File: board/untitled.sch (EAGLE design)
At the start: 32 parts, among them IC1 PIC16F628P, IC2 LP2950CZ-3.3, Q1 BC546B, Q2 BC546B

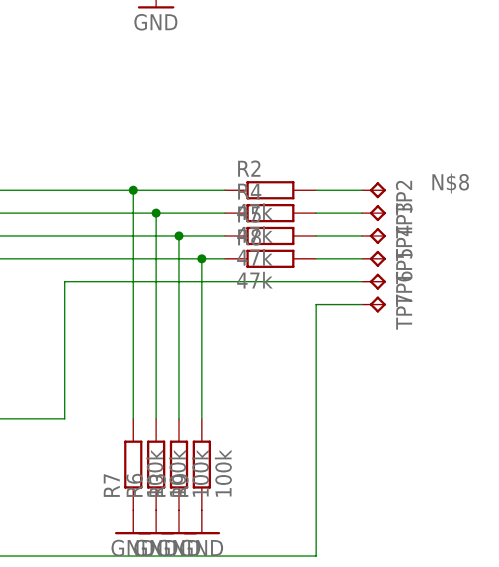
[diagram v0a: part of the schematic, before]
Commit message: - Added notes
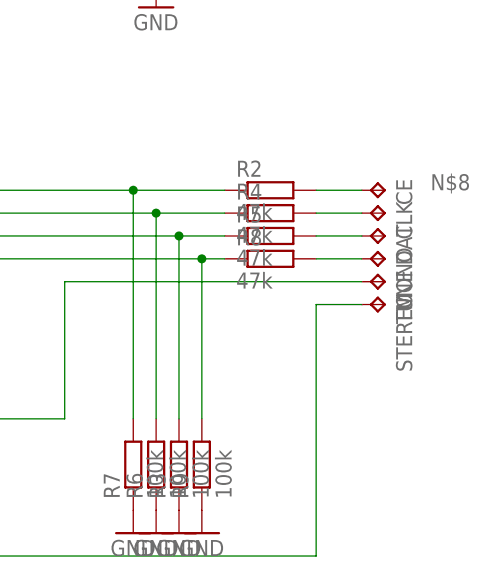
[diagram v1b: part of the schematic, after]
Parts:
- renumbered TP2 to CE, TP3 to CLK, TP4 to DAT, TP5 to MONO, TP6 to TUNE, TP7 to STEREO
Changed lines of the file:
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@@
 <part name="R13" library="rcl" library_urn="urn:adsk.eagle:library:334" deviceset="R-EU_" device="0204/7" package3d_urn="urn:adsk.eagle:package:23498/2" value="10k"/>
 <part name="P+3" library="supply1" library_urn="urn:adsk.eagle:library:371" deviceset="+5V" device=""/>
-<part name="TP2" library="testpad" library_urn="urn:adsk.eagle:library:385" deviceset="TP" device="B1,27" package3d_urn="urn:adsk.eagle:package:27944/2"/>
-<part name="TP3" library="testpad" library_urn="urn:adsk.eagle:library:385" deviceset="TP" device="B1,27" package3d_urn="urn:adsk.eagle:package:27944/2"/>
-<part name="TP4" library="testpad" library_urn="urn:adsk.eagle:library:385" deviceset="TP" device="B1,27" package3d_urn="urn:adsk.eagle:package:27944/2"/>
-<part name="TP5" library="testpad" library_urn="urn:adsk.eagle:library:385" deviceset="TP" device="B1,27" package3d_urn="urn:adsk.eagle:package:27944/2"/>
-<part name="TP6" library="testpad" library_urn="urn:adsk.eagle:library:385" deviceset="TP" device="B1,27" package3d_urn="urn:adsk.eagle:package:27944/2"/>
-<part name="TP7" library="testpad" library_urn="urn:adsk.eagle:library:385" deviceset="TP" device="B1,27" package3d_urn="urn:adsk.eagle:package:27944/2"/>
+<part name="CE" library="testpad" library_urn="urn:adsk.eagle:library:385" deviceset="TP" device="B1,27" package3d_urn="urn:adsk.eagle:package:27944/2"/>
+<part name="CLK" library="testpad" library_urn="urn:adsk.eagle:library:385" deviceset="TP" device="B1,27" package3d_urn="urn:adsk.eagle:package:27944/2"/>
+<part name="DAT" library="testpad" library_urn="urn:adsk.eagle:library:385" deviceset="TP" device="B1,27" package3d_urn="urn:adsk.eagle:package:27944/2"/>
+<part name="MONO" library="testpad" library_urn="urn:adsk.eagle:library:385" deviceset="TP" device="B1,27" package3d_urn="urn:adsk.eagle:package:27944/2"/>
+<part name="TUNE" library="testpad" library_urn="urn:adsk.eagle:library:385" deviceset="TP" device="B1,27" package3d_urn="urn:adsk.eagle:package:27944/2"/>
+<part name="STEREO" library="testpad" library_urn="urn:adsk.eagle:library:385" deviceset="TP" device="B1,27" package3d_urn="urn:adsk.eagle:package:27944/2"/>
 <part name="TP8" library="testpad" library_urn="urn:adsk.eagle:library:385" deviceset="TP" device="B1,27" package3d_urn="urn:adsk.eagle:package:27944/2"/>
 <part name="TP9" library="testpad" library_urn="urn:adsk.eagle:library:385" deviceset="TP" device="B1,27" package3d_urn="urn:adsk.eagle:package:27944/2"/>
@@
 <attribute name="VALUE" x="60.96" y="7.62" size="1.778" layer="96" rot="R90"/>
 </instance>
-<instance part="TP2" gate="G$1" x="129.54" y="25.4" smashed="yes" rot="R270">
+<instance part="CE" gate="G$1" x="129.54" y="25.4" smashed="yes" rot="R270">
 <attribute name="NAME" x="130.81" y="26.67" size="1.778" layer="95" rot="R270"/>
 <attribute name="TP_SIGNAL_NAME" x="128.27" y="24.13" size="1.778" layer="97" rot="R270"/>
 </instance>
-<instance part="TP3" gate="G$1" x="129.54" y="22.86" smashed="yes" rot="R270">
+<instance part="CLK" gate="G$1" x="129.54" y="22.86" smashed="yes" rot="R270">
 <attribute name="NAME" x="130.81" y="24.13" size="1.778" layer="95" rot="R270"/>
 <attribute name="TP_SIGNAL_NAME" x="128.27" y="21.59" size="1.778" layer="97" rot="R270"/>
 </instance>
-<instance part="TP4" gate="G$1" x="129.54" y="20.32" smashed="yes" rot="R270">
+<instance part="DAT" gate="G$1" x="129.54" y="20.32" smashed="yes" rot="R270">
 <attribute name="NAME" x="130.81" y="21.59" size="1.778" layer="95" rot="R270"/>
 <attribute name="TP_SIGNAL_NAME" x="128.27" y="19.05" size="1.778" layer="97" rot="R270"/>
 </instance>
-<instance part="TP5" gate="G$1" x="129.54" y="17.78" smashed="yes" rot="R270">
+<instance part="MONO" gate="G$1" x="129.54" y="17.78" smashed="yes" rot="R270">
 <attribute name="NAME" x="130.81" y="19.05" size="1.778" layer="95" rot="R270"/>
 <attribute name="TP_SIGNAL_NAME" x="128.27" y="16.51" size="1.778" layer="97" rot="R270"/>
 </instance>
-<instance part="TP6" gate="G$1" x="129.54" y="15.24" smashed="yes" rot="R270">
+<instance part="TUNE" gate="G$1" x="129.54" y="15.24" smashed="yes" rot="R270">
 <attribute name="NAME" x="130.81" y="16.51" size="1.778" layer="95" rot="R270"/>
 <attribute name="TP_SIGNAL_NAME" x="128.27" y="13.97" size="1.778" layer="97" rot="R270"/>
 </instance>
-<instance part="TP7" gate="G$1" x="129.54" y="12.7" smashed="yes" rot="R270">
+<instance part="STEREO" gate="G$1" x="129.54" y="12.7" smashed="yes" rot="R270">
 <attribute name="NAME" x="130.81" y="13.97" size="1.778" layer="95" rot="R270"/>
 <attribute name="TP_SIGNAL_NAME" x="128.27" y="11.43" size="1.778" layer="97" rot="R270"/>
@@
 <wire x1="127" y1="25.4" x2="121.92" y2="25.4" width="0.1524" layer="91"/>
 <label x="134.62" y="25.4" size="1.778" layer="95"/>
-<pinref part="TP2" gate="G$1" pin="TP"/>
+<pinref part="CE" gate="G$1" pin="TP"/>
 </segment>
 </net>
@@
 <pinref part="R4" gate="G$1" pin="2"/>
 <wire x1="121.92" y1="22.86" x2="127" y2="22.86" width="0.1524" layer="91"/>
-<pinref part="TP3" gate="G$1" pin="TP"/>
+<pinref part="CLK" gate="G$1" pin="TP"/>
 </segment>
 </net>
@@
 <pinref part="R5" gate="G$1" pin="2"/>
 <wire x1="127" y1="20.32" x2="121.92" y2="20.32" width="0.1524" layer="91"/>
-<pinref part="TP4" gate="G$1" pin="TP"/>
+<pinref part="DAT" gate="G$1" pin="TP"/>
 </segment>
 </net>
@@
 <pinref part="R8" gate="G$1" pin="2"/>
 <wire x1="121.92" y1="17.78" x2="127" y2="17.78" width="0.1524" layer="91"/>
-<pinref part="TP5" gate="G$1" pin="TP"/>
+<pinref part="MONO" gate="G$1" pin="TP"/>
 </segment>
 </net>
@@
 <wire x1="93.98" y1="0" x2="78.74" y2="0" width="0.1524" layer="91"/>
 <junction x="78.74" y="0"/>
-<pinref part="TP6" gate="G$1" pin="TP"/>
+<pinref part="TUNE" gate="G$1" pin="TP"/>
 </segment>
 </net>
@@
 <wire x1="121.92" y1="-15.24" x2="121.92" y2="12.7" width="0.1524" layer="91"/>
 <wire x1="121.92" y1="12.7" x2="127" y2="12.7" width="0.1524" layer="91"/>
-<pinref part="TP7" gate="G$1" pin="TP"/>
-</segment>
-</net>
+<pinref part="STEREO" gate="G$1" pin="TP"/>
+</segment>
+</net>
